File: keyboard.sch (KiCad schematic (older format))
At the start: 30 parts, among them J1 USB_OTG, K1 Jumper_NO_Small, P1 SWD, P2 BATT, U1 nrf51822-02, U2 CH554T, U3 TP4057, U4 RT9193

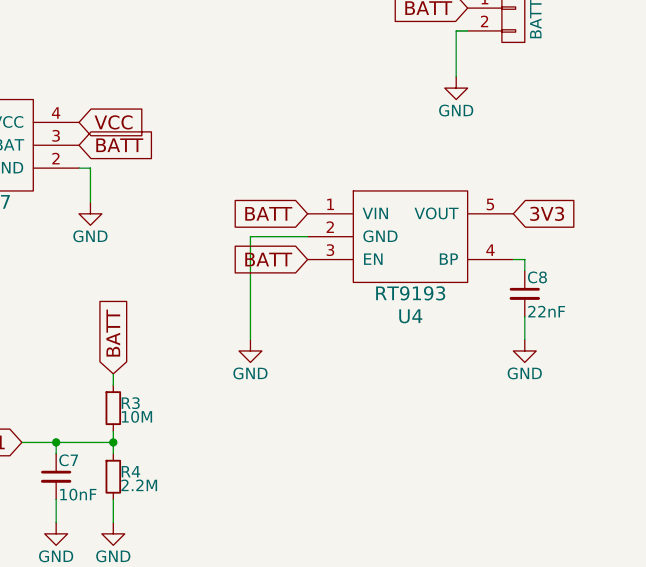
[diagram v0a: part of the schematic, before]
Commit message: 修改
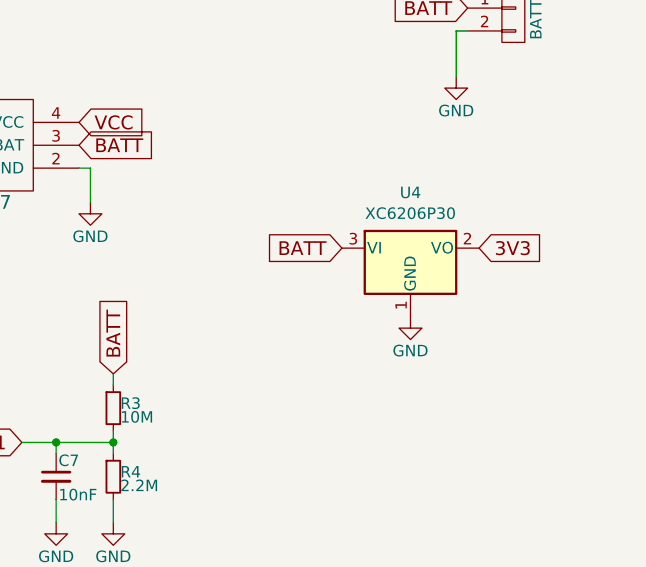
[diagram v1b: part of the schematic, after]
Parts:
- removed C8: 22nF, Capacitor_SMD:C_0805_2012Metric, symbol keyboard-rescue:C_Small-RESCUE-ble4100-nrf-ble4100-nrf-rescue
- removed U4: RT9193, Package_TO_SOT_SMD:SOT-23-5, symbol keyboard-rescue:RT9193-RESCUE-ble4100-nrf-ble4100-nrf-rescue
- added U4: XC6206P30, Package_TO_SOT_SMD:SOT-23, symbol Regulator_Linear:AP2127N-3.0
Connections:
- wire segments 109 -> 104
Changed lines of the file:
@@
-$EndComp
-$Comp
-L keyboard-rescue:RT9193-RESCUE-ble4100-nrf-ble4100-nrf-rescue U4
-U 1 1 58687662
-P 10250 4850
-F 0 "U4" H 10250 4650 60  0000 C CNN
-F 1 "RT9193" H 10250 4750 60  0000 C CNN
-F 2 "Package_TO_SOT_SMD:SOT-23-5" H 10200 4850 60  0001 C CNN
-F 3 "" H 10200 4850 60  0001 C CNN
-	1    10250 4850
-	1    0    0    -1
 $EndComp
 $Comp
@@
 Text GLabel 8800 4300 2    60   Input ~ 0
 BATT
-Text GLabel 9800 4600 0    60   Input ~ 0
-BATT
 Text GLabel 10500 3700 0    60   Input ~ 0
 BATT
-$Comp
-L keyboard-rescue:GND-RESCUE-ble4100-nrf-ble4100-nrf-rescue #PWR016
-U 1 1 5868900A
-P 9550 5150
-F 0 "#PWR016" H 9550 4900 50  0001 C CNN
-F 1 "GND" H 9550 5000 50  0000 C CNN
-F 2 "" H 9550 5150 50  0000 C CNN
-F 3 "" H 9550 5150 50  0000 C CNN
-	1    9550 5150
-	1    0    0    -1
-$EndComp
-Text GLabel 10700 4600 2    60   Input ~ 0
-3V3
 Text GLabel 1750 4500 2    60   Input ~ 0
 3V3
@@
 DCLK
 $Comp
-L keyboard-rescue:C_Small-RESCUE-ble4100-nrf-ble4100-nrf-rescue C8
-U 1 1 58689C31
-P 10750 4950
-F 0 "C8" H 10760 5020 50  0000 L CNN
-F 1 "22nF" H 10760 4870 50  0000 L CNN
-F 2 "Capacitor_SMD:C_0805_2012Metric" H 10750 4950 50  0001 C CNN
-F 3 "" H 10750 4950 50  0000 C CNN
-	1    10750 4950
-	1    0    0    -1
-$EndComp
-$Comp
 L Device:C_Small C5
 U 1 1 58689C6E
@@
 F 3 "" H 8100 5750 50  0000 C CNN
 	1    8100 5750
-	1    0    0    -1
-$EndComp
-$Comp
-L keyboard-rescue:GND-RESCUE-ble4100-nrf-ble4100-nrf-rescue #PWR018
-U 1 1 5868A007
-P 10750 5150
-F 0 "#PWR018" H 10750 4900 50  0001 C CNN
-F 1 "GND" H 10750 5000 50  0000 C CNN
-F 2 "" H 10750 5150 50  0000 C CNN
-F 3 "" H 10750 5150 50  0000 C CNN
-	1    10750 5150
 	1    0    0    -1
 $EndComp
@@
 	10450 3800 10450 4000
 Wire Wire Line
-	9800 4700 9550 4700
-Wire Wire Line
 	1750 4200 1850 4200
 Wire Wire Line
@@
 Connection ~ 1550 2850
 Wire Wire Line
-	10700 4800 10750 4800
-Wire Wire Line
 	7850 4400 7900 4400
 Wire Wire Line
 	7650 5850 7650 5950
-Wire Wire Line
-	9550 4700 9550 5150
 Wire Wire Line
 	7650 4400 7550 4400
@@
 	8950 5350 8950 5300
 Connection ~ 8700 5600
-Wire Wire Line
-	10750 4800 10750 4850
-Wire Wire Line
-	10750 5050 10750 5150
 Wire Notes Line
 	7300 2700 11200 2700
@@
 	8000 5900 8000 5950
 Connection ~ 8000 5900
-Text GLabel 9800 4800 0    60   Input ~ 0
-BATT
 $Comp
 L keyboard-rescue:CH554T-ch554t U2
@@
 	3550 2650 3850 2650
 NoConn ~ 2900 3200
+$Comp
+L Regulator_Linear:AP2127N-3.0 U4
+U 1 1 5AE6D677
+P 10250 4750
+F 0 "U4" H 10250 4992 50  0000 C CNN
+F 1 "XC6206P30" H 10250 4901 50  0000 C CNN
+F 2 "Package_TO_SOT_SMD:SOT-23" H 10250 4975 50  0001 C CIN
+F 3 "https://www.diodes.com/assets/Datasheets/AP2127.pdf" H 10250 4750 50  0001 C CNN
+	1    10250 4750
+	1    0    0    -1
+$EndComp
+Text GLabel 9950 4750 0    60   Input ~ 0
+BATT
+Text GLabel 10550 4750 2    60   Input ~ 0
+3V3
+$Comp
+L keyboard-rescue:GND-RESCUE-ble4100-nrf-ble4100-nrf-rescue #PWR016
+U 1 1 5AE6D8BF
+P 10250 5050
+F 0 "#PWR016" H 10250 4800 50  0001 C CNN
+F 1 "GND" H 10250 4900 50  0000 C CNN
+F 2 "" H 10250 5050 50  0000 C CNN
+F 3 "" H 10250 5050 50  0000 C CNN
+	1    10250 5050
+	1    0    0    -1
+$EndComp
 Wire Bus Line
 	1200 3500 3950 3500
